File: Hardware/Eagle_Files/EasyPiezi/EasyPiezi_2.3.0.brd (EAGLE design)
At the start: 43 x 15.4 mm, 72 parts, among them J1 CON-MOLEX-6P-1.25MM048, U2 LM317DCYSOT89, U3 LM2902QT, U4 ATMEGA48/88/168/328PB

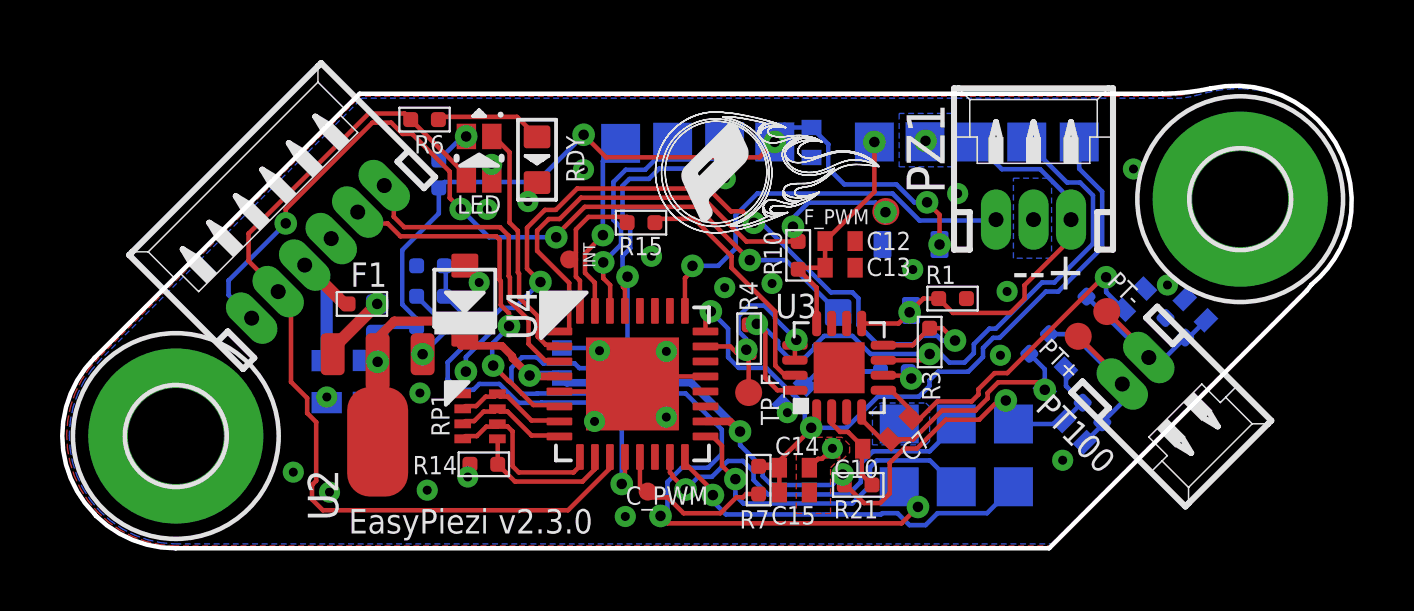
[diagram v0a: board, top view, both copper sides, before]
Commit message: fixed component values and names for v2.3.0 #bugfix
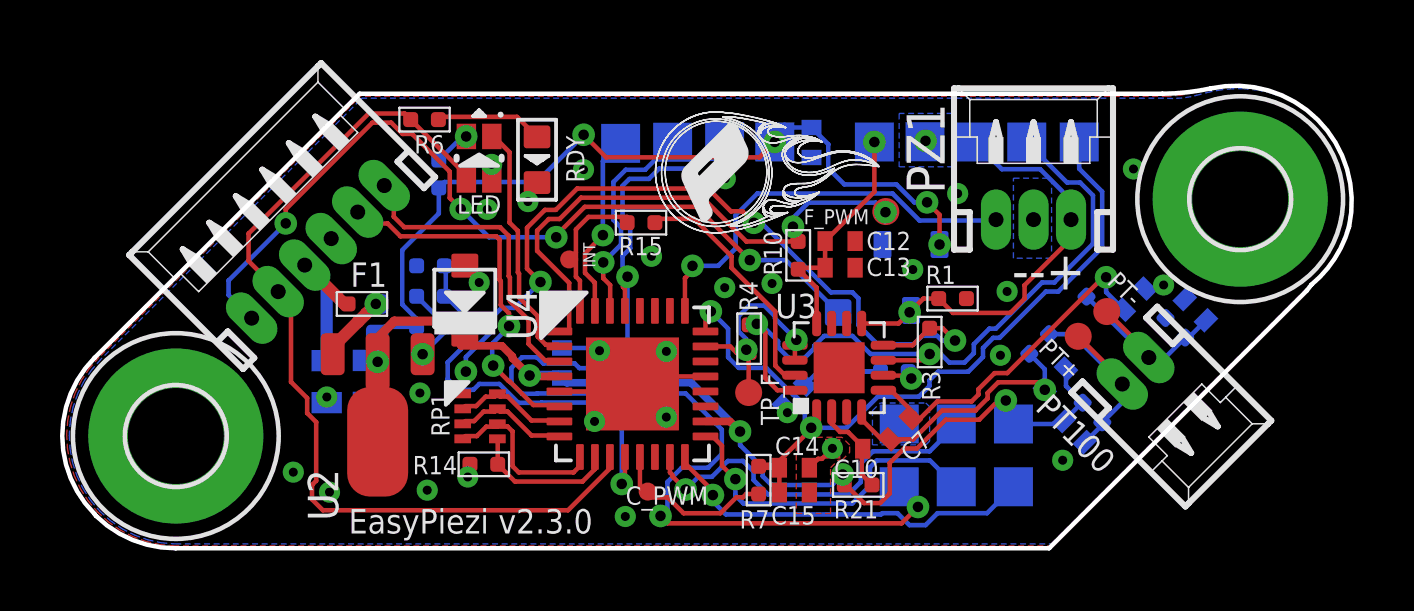
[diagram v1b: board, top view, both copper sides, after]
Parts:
- R2: value (none) -> 2K2
- R5: value (none) -> 3K
- R9: value (none) -> 3K6
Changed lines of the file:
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@@
 </layers>
 <board>
-<fusionsync huburn="a.cGVyc29uYWw6dWUyYTEyMDdh" projecturn="a.cGVyc29uYWw6dWUyYTEyMDdhIzIwMTgxMTI5MTYyOTY3NjMx" f3durn="urn:adsk.wipprod:dm.lineage:169Sjry_R56h3jRKqfc0NQ" pcbguid="6fe6201e-d7cf-425a-9275-8c8c67dd0b6c" lastpulledtime="" lastsyncedchangeguid="bb61cdab-da3f-cf89-6c5e-13e2484f2520"/>
+<fusionsync huburn="a.cGVyc29uYWw6dWUyYTEyMDdh" projecturn="a.cGVyc29uYWw6dWUyYTEyMDdhIzIwMTgxMTI5MTYyOTY3NjMx" f3durn="urn:adsk.wipprod:dm.lineage:78mEL7qyToiMJn8ubwKObw" pcbguid="360ab3a3-11fc-4ca8-a52a-227fd8b2059a" lastpulledtime="" lastsyncedchangeguid="534f509e-7677-5851-aa15-9bb12285179b"/>
 <plain>
 <text x="34.778753125" y="9.75258125" size="1.27" layer="22" ratio="11" rot="R180">--+</text>
@@
 </element>
 <element name="C4" library="PiezoFFC" library_urn="urn:adsk.eagle:library:6897166" package="CAPC1005X50" package3d_urn="urn:adsk.eagle:package:5248669/4" value="0.1uF" x="17.3355" y="6.0325" smashed="yes" rot="MR270">
-<attribute name="NAME" x="17.3355" y="7.4831" size="0.6096" layer="26" font="vector" ratio="11" rot="MR180" align="bottom-center"/>
+<attribute name="NAME" x="17.3355" y="7.4831" size="0.8128" layer="26" font="vector" ratio="11" rot="MR180" align="bottom-center"/>
 </element>
 <element name="U3" library="PiezoFFC" library_urn="urn:adsk.eagle:library:6897166" package="QFN16" package3d_urn="urn:adsk.eagle:package:8766128/2" value="LM2902QT" x="26.57475" y="5.87375" smashed="yes" rot="R90">
@@
 <attribute name="VALUE" x="19.939" y="1.36525" size="0.0254" layer="27"/>
 </element>
-<element name="R2" library="PiezoFFC" library_urn="urn:adsk.eagle:library:6897166" package="R0402" package3d_urn="urn:adsk.eagle:package:7115182/2" value="" x="12.954" y="7.239" smashed="yes" rot="MR90">
+<element name="R2" library="PiezoFFC" library_urn="urn:adsk.eagle:library:6897166" package="R0402" package3d_urn="urn:adsk.eagle:package:7115182/2" value="2K2" x="12.954" y="7.239" smashed="yes" rot="MR90">
 <attribute name="MPN" value="RC0402JR-070RL" x="18.034" y="4.191" size="1.778" layer="28" rot="MR90" display="off"/>
-<attribute name="NAME" x="14.224" y="7.874" size="0.8128" layer="26" font="vector" ratio="11" rot="MR0"/>
+<attribute name="NAME" x="14.097" y="7.62" size="0.8128" layer="26" font="vector" ratio="11" rot="MR180"/>
 <attribute name="VALUE" x="14.224" y="5.715" size="0.8128" layer="28" font="vector" ratio="11" rot="MR0"/>
 </element>
-<element name="R5" library="PiezoFFC" library_urn="urn:adsk.eagle:library:6897166" package="R0402" package3d_urn="urn:adsk.eagle:package:7115182/2" value="" x="12.954" y="8.255" smashed="yes" rot="MR90">
+<element name="R5" library="PiezoFFC" library_urn="urn:adsk.eagle:library:6897166" package="R0402" package3d_urn="urn:adsk.eagle:package:7115182/2" value="3K" x="12.954" y="8.255" smashed="yes" rot="MR90">
 <attribute name="MPN" value="RC0402JR-070RL" x="17.907" y="5.207" size="1.778" layer="28" rot="MR90" display="off"/>
-<attribute name="NAME" x="13.97" y="8.636" size="0.8128" layer="26" font="vector" ratio="11" rot="MR180"/>
+<attribute name="NAME" x="14.097" y="8.636" size="0.8128" layer="26" font="vector" ratio="11" rot="MR180"/>
 <attribute name="VALUE" x="14.224" y="6.731" size="0.8128" layer="28" font="vector" ratio="11" rot="MR0"/>
 </element>
-<element name="R9" library="PiezoFFC" library_urn="urn:adsk.eagle:library:6897166" package="R0402" package3d_urn="urn:adsk.eagle:package:7115182/2" value="" x="12.954" y="9.271" smashed="yes" rot="MR270">
+<element name="R9" library="PiezoFFC" library_urn="urn:adsk.eagle:library:6897166" package="R0402" package3d_urn="urn:adsk.eagle:package:7115182/2" value="3K6" x="12.954" y="9.271" smashed="yes" rot="MR270">
 <attribute name="MPN" value="RC0402JR-070RL" x="8.001" y="12.319" size="1.778" layer="28" rot="MR270" display="off"/>
-<attribute name="NAME" x="13.97" y="9.652" size="0.8128" layer="26" font="vector" ratio="11" rot="MR180"/>
+<attribute name="NAME" x="13.97" y="9.779" size="0.8128" layer="26" font="vector" ratio="11" rot="MR180"/>
 <attribute name="VALUE" x="11.684" y="10.795" size="0.8128" layer="28" font="vector" ratio="11" rot="MR180"/>
 </element>
@@
 <wire x1="25.5825" y1="2.54" x2="25.5825" y2="2.546075" width="0.1524" layer="1"/>
 <via x="29.0302125" y="9.147590625" extent="1-16" drill="0.3"/>
-<via x="37.517534375" y="8.632065625" extent="1-16" drill="0.3"/>
+<via x="37.390534375" y="8.632065625" extent="1-16" drill="0.3"/>
 <contactref element="D8" pad="1"/>
 <contactref element="U4" pad="5"/>
@@
 <wire x1="9.692796875" y1="6.3255" x2="9.692796875" y2="6.563296875" width="0.4064" layer="1"/>
 <wire x1="9.692796875" y1="6.3255" x2="9.692796875" y2="6.517796875" width="0.4064" layer="1"/>
-<wire x1="9.692796875" y1="6.517796875" x2="11.176" y2="8.001" width="0.4064" layer="1"/>
-<via x="11.176" y="8.001" extent="1-16" drill="0.35"/>
-<wire x1="11.176" y1="8.001" x2="11.1305" y2="8.001" width="0" layer="19" extent="1-16"/>
+<wire x1="9.692796875" y1="6.563296875" x2="10.5249" y2="7.3954" width="0.4064" layer="1"/>
+<wire x1="10.5249" y1="7.3954" x2="10.52956875" y2="7.3954" width="0.4064" layer="1"/>
+<wire x1="10.52956875" y1="7.3954" x2="10.8111" y2="7.67693125" width="0.4064" layer="1"/>
+<wire x1="10.8111" y1="7.67693125" x2="10.8111" y2="7.6816" width="0.4064" layer="1"/>
+<wire x1="10.8111" y1="7.6816" x2="11.1305" y2="8.001" width="0.4064" layer="1"/>
+<wire x1="11.176" y1="8.001" x2="11.1305" y2="8.001" width="0.1524" layer="16"/>
+<via x="11.1305" y="8.001" extent="1-16" drill="0.35"/>
 </signal>
 <signal name="AMP_VCC">
